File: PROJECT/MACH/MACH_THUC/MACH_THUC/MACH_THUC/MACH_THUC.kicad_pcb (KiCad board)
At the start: 2 copper layers, 204.5 x 138.6 mm, 65 parts, among them K1 SANYOU_SRD_Form_C, K2 SANYOU_SRD_Form_C, Q1 2SB688, Q2 BC547, Q3 BC547, U1 LM7805_TO220, U2 DS1307+, U3 LCD-016N002L, U4 PCF8574, U5 PC817, U6 PC817, Y1 Crystal 20M, Y2 Crystal 32.768KHz

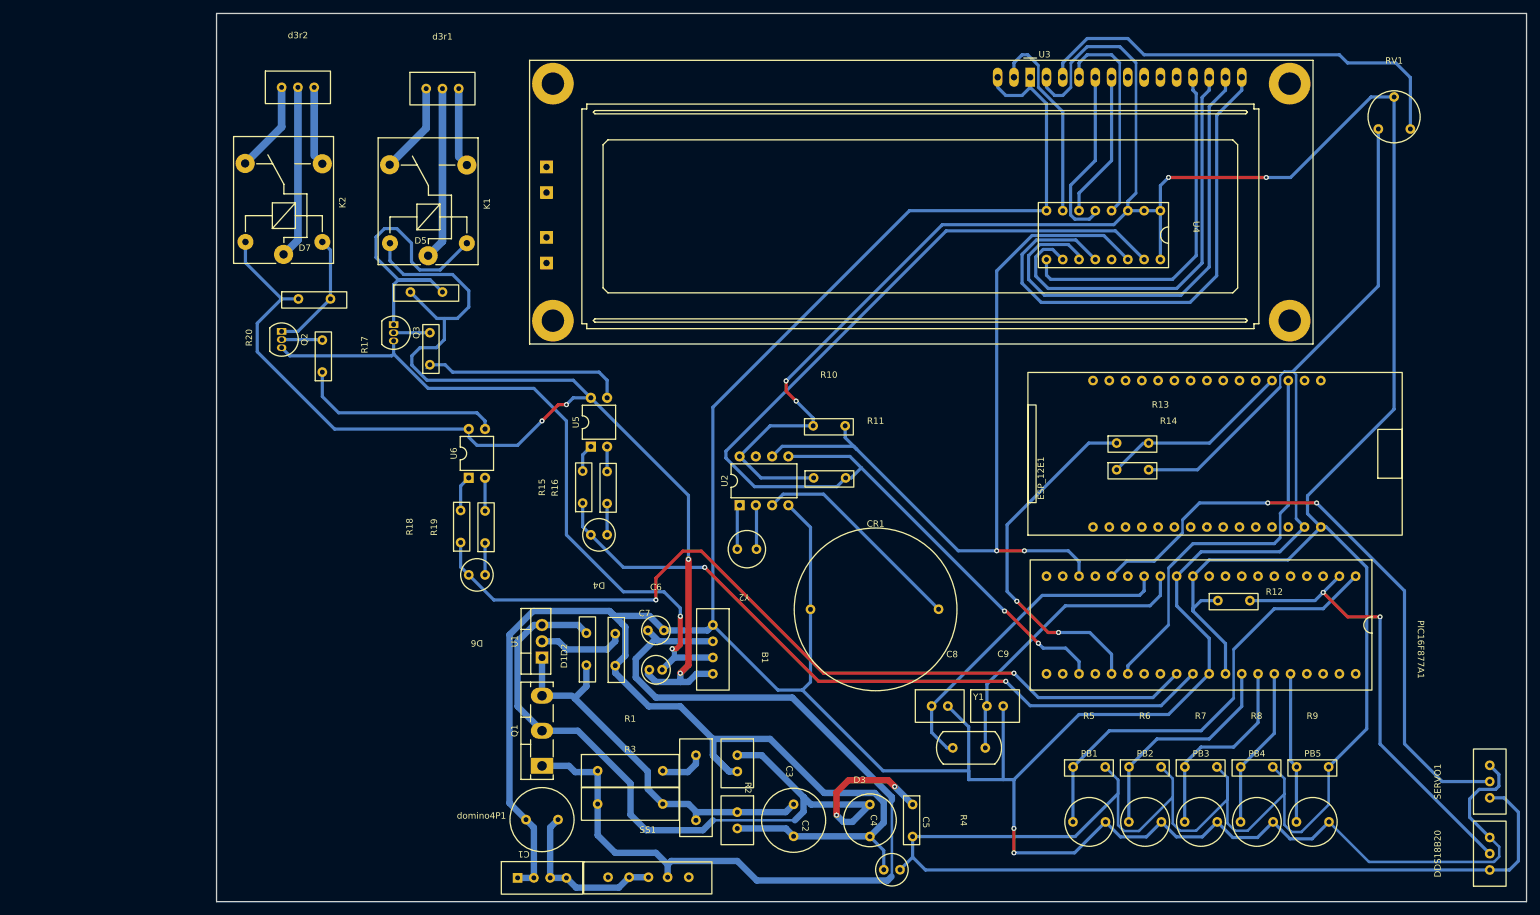
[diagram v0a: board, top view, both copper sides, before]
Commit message: update code
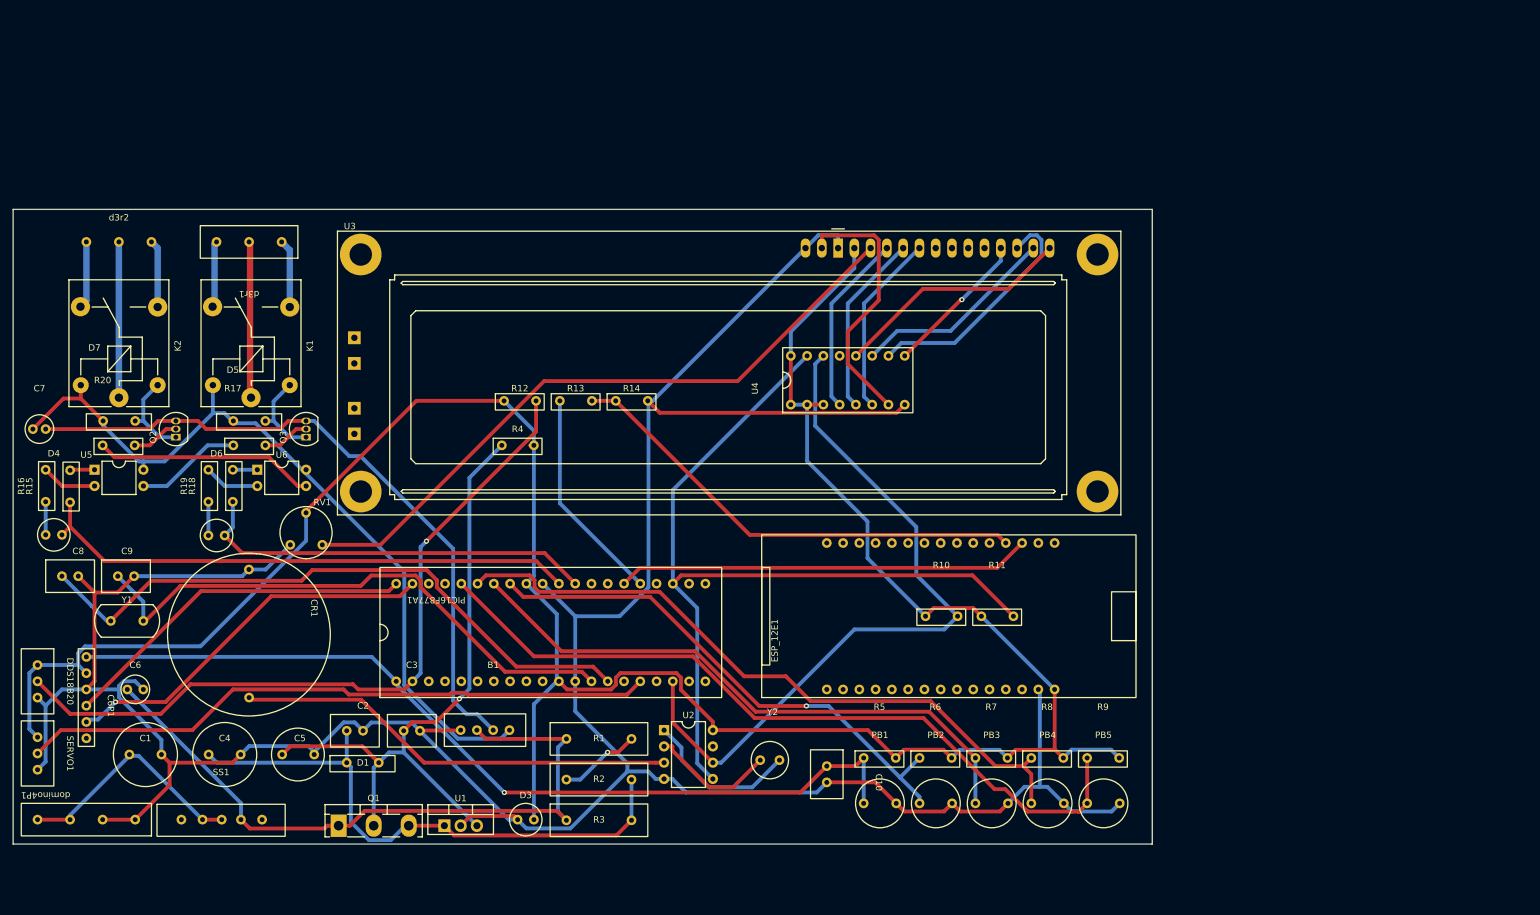
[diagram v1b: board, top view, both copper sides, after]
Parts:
- removed D2: 1N4007, library_thuan_footprint:1N4007
- added C10: 100nF, library_thuan_footprint:CAP_104, F.Cu at (174.0, 140.2)
- added C6P1: ~, library_thuan_footprint:CONNECT_6PIN, F.Cu at (61.0, 128.3)
- C8, C9: value 33pF -> 22pF
- d3r1: footprint library_thuan_footprint:DOMINO_3 -> library_thuan_footprint:DOMINO_3_5mm
- d3r2: footprint library_thuan_footprint:DOMINO_3 -> library_thuan_footprint:DOMINO_3_5mm; moved to B.Cu
- domino4P1: footprint library_thuan_footprint:DOMINO_4 -> library_thuan_footprint:DOMINO_4_5mm
- moved DDS18B20 213.1 mm to (50.8, 124.5), turned to -90 degrees
- moved SERVO1 211.5 mm to (50.8, 135.7), turned to -90 degrees
- moved RV1 181.8 mm to (85.1, 93.0)
- moved PIC16F877A1 160.1 mm to (94.1, 113.0), turned to 90 degrees
- moved C8 137.2 mm to (49.5, 100.4)
- moved C9 137.2 mm to (58.2, 100.4)
- moved Y1 132.9 mm to (57.1, 108.7)
- moved R12 115.7 mm to (118.5, 73.2)
- moved C7 103.3 mm to (43.5, 79.2)
- moved C5 99.0 mm to (84.1, 127.6), turned to 0 degrees
- moved R4 95.6 mm to (118.1, 80.2), turned to 0 degrees
- moved C4 95.0 mm to (72.4, 130.9), turned to 0 degrees
- moved R16 87.6 mm to (37.0, 94.0)
- moved D4 87.5 mm to (45.7, 91.4), turned to 0 degrees
- moved R13 87.2 mm to (127.2, 73.2)
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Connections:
- PIC16F877A1 pad 39: unconnected-(PIC16F877A1-RB6-Pad39) -> pgc
- PIC16F877A1 pad 40: unconnected-(PIC16F877A1-RB7-Pad40) ->  pgd
- U1 pad 2: Net-(D2-A) -> GND1
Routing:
- net GND1: track 723.4 -> 478.6 mm, vias 2 -> 0
- net +5V: track 614.7 -> 391.0 mm, vias 4 -> 0
- net +5P: track 222.0 -> 124.8 mm, vias 4 -> 0
- net btn_4: track 23.5 -> 120.0 mm
- net btn_3: track 25.3 -> 106.8 mm
- net relay_2: track 133.9 -> 63.6 mm, vias 2 -> 0
- net rst: track 69.5 -> 139.7 mm, vias 0 -> 1
- net btn_2: track 30.8 -> 93.5 mm
- net pgc: track 0.00 -> 60.1 mm, vias 0 -> 1
- net  pgd: track 0.00 -> 56.4 mm
- net osc2: track 51.3 -> 99.2 mm
- net btn_1: track 35.2 -> 83.0 mm, vias 0 -> 1
- net Net-(U3-DB7): track 84.1 -> 37.2 mm
- net ds_18b20: track 70.1 -> 115.2 mm, vias 2 -> 1
- net Net-(ESP_12E1-RX): track 30.0 -> 73.8 mm
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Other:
- board size 204.5 x 138.6 mm -> 177.8 x 99.1 mm
